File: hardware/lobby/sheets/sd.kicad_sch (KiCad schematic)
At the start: 8 parts, among them J3 Micro_SD_Card_Det, U1 RT9742GGJ5

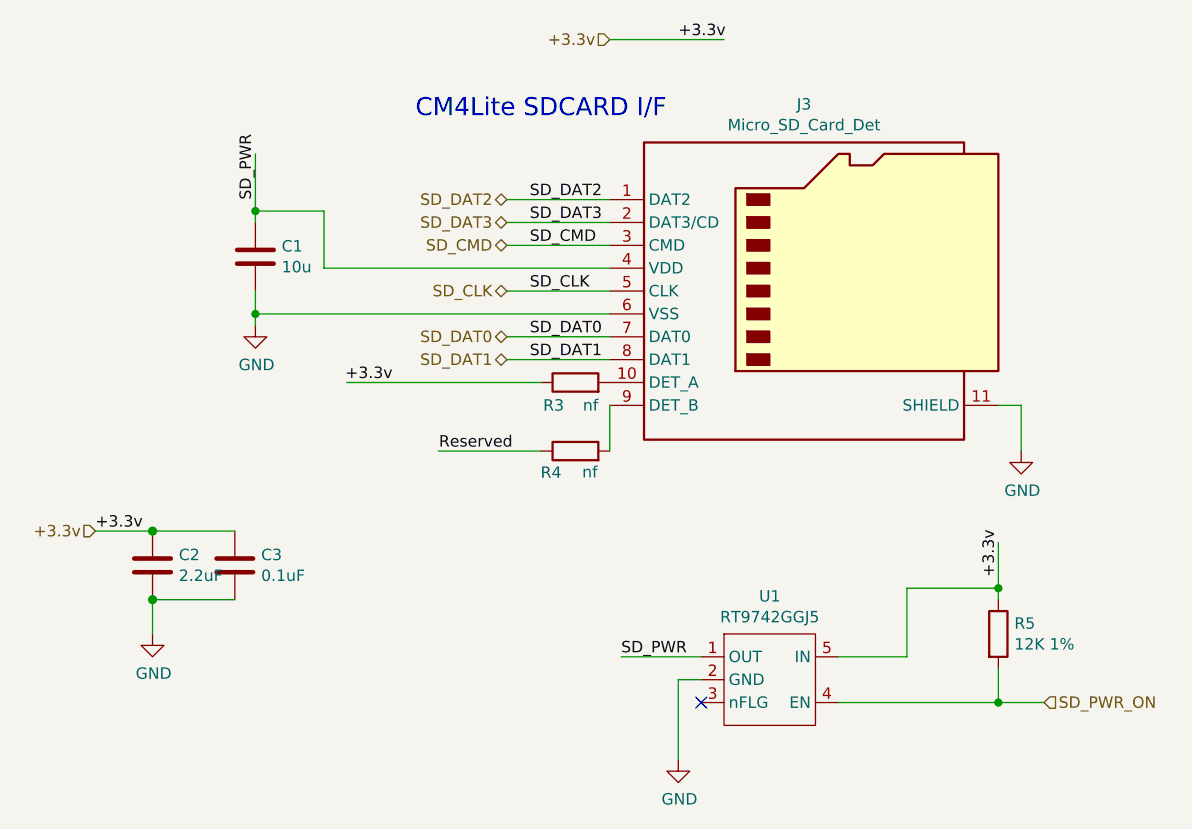
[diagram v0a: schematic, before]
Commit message: update lobby
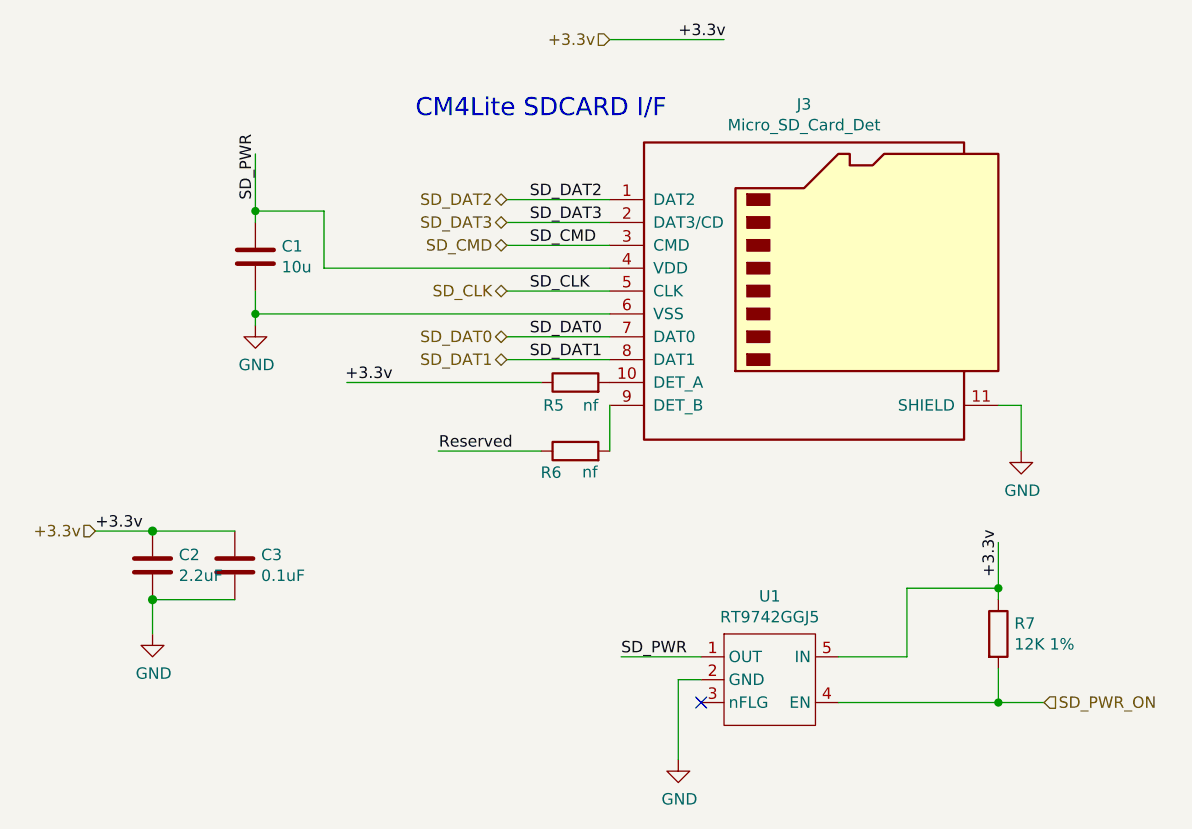
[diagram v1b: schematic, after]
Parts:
- J3: footprint cm4crypto:SDCARD_MOLEX_503398-1892 -> cm4crypto:amphenol-sd-push-pull_114-00841-68
- renumbered R3 to R5, R4 to R6, R5 to R7
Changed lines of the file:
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@@
   (symbol (lib_id "power:GND") (at 86.36 119.38 0) (unit 1)
     (in_bom yes) (on_board yes)
-    (property "Reference" "#PWR056" (id 0) (at 86.36 125.73 0)
+    (property "Reference" "#PWR055" (id 0) (at 86.36 125.73 0)
       (effects (font (size 1.27 1.27)) hide)
     )
@@
   (symbol (lib_id "power:GND") (at 97.79 85.09 0) (unit 1)
     (in_bom yes) (on_board yes)
-    (property "Reference" "#PWR054" (id 0) (at 97.79 91.44 0)
+    (property "Reference" "#PWR053" (id 0) (at 97.79 91.44 0)
       (effects (font (size 1.27 1.27)) hide)
     )
@@
   (symbol (lib_id "power:GND") (at 144.78 133.35 0) (unit 1)
     (in_bom yes) (on_board yes)
-    (property "Reference" "#PWR057" (id 0) (at 144.78 139.7 0)
+    (property "Reference" "#PWR056" (id 0) (at 144.78 139.7 0)
       (effects (font (size 1.27 1.27)) hide)
     )
@@
   (symbol (lib_id "power:GND") (at 182.88 99.06 0) (unit 1)
     (in_bom yes) (on_board yes)
-    (property "Reference" "#PWR055" (id 0) (at 182.88 105.41 0)
+    (property "Reference" "#PWR054" (id 0) (at 182.88 105.41 0)
       (effects (font (size 1.27 1.27)) hide)
     )
@@
   (symbol (lib_id "Device:R") (at 133.35 91.44 90) (unit 1)
     (in_bom yes) (on_board yes)
-    (property "Reference" "R3" (id 0) (at 132.08 93.98 90)
+    (property "Reference" "R5" (id 0) (at 132.08 93.98 90)
       (effects (font (size 1.27 1.27)) (justify left))
     )
@@
       (effects (font (size 1.27 1.27)) hide)
     )
-    (property "Datasheet" "https://fscdn.rohm.com/en/products/databook/datasheet/passive/resistor/chip_resistor/mcr-e.pdf" (id 3) (at 133.35 91.44 0)
+    (property "Datasheet" "~" (id 3) (at 133.35 91.44 0)
       (effects (font (size 1.27 1.27)) hide)
     )
@@
   (symbol (lib_id "Device:R") (at 133.35 99.06 90) (unit 1)
     (in_bom yes) (on_board yes)
-    (property "Reference" "R4" (id 0) (at 131.8006 101.4476 90)
+    (property "Reference" "R6" (id 0) (at 131.8006 101.4476 90)
       (effects (font (size 1.27 1.27)) (justify left))
     )
@@
       (effects (font (size 1.27 1.27)) hide)
     )
-    (property "Datasheet" "https://fscdn.rohm.com/en/products/databook/datasheet/passive/resistor/chip_resistor/mcr-e.pdf" (id 3) (at 133.35 99.06 0)
+    (property "Datasheet" "~" (id 3) (at 133.35 99.06 0)
       (effects (font (size 1.27 1.27)) hide)
     )
@@
   (symbol (lib_id "Device:R") (at 180.34 119.38 0) (unit 1)
     (in_bom yes) (on_board yes)
-    (property "Reference" "R5" (id 0) (at 182.118 118.2116 0)
+    (property "Reference" "R7" (id 0) (at 182.118 118.2116 0)
       (effects (font (size 1.27 1.27)) (justify left))
     )
@@
       (effects (font (size 1.27 1.27)) hide)
     )
-    (property "Datasheet" "https://fscdn.rohm.com/en/products/databook/datasheet/passive/resistor/chip_resistor/mcr-e.pdf" (id 3) (at 180.34 119.38 0)
+    (property "Datasheet" "~" (id 3) (at 180.34 119.38 0)
       (effects (font (size 1.27 1.27)) hide)
     )
@@
       (effects (font (size 1.27 1.27)) hide)
     )
-    (property "Datasheet" "https://search.murata.co.jp/Ceramy/image/img/A01X/G101/ENG/GRM21BR71A106KA73-01.pdf" (id 3) (at 86.36 111.76 0)
+    (property "Datasheet" "~" (id 3) (at 86.36 111.76 0)
       (effects (font (size 1.27 1.27)) hide)
     )
@@
       (effects (font (size 1.27 1.27)) hide)
     )
-    (property "Datasheet" "https://search.murata.co.jp/Ceramy/image/img/A01X/G101/ENG/GRM21BR71A106KA73-01.pdf" (id 3) (at 95.504 111.76 0)
+    (property "Datasheet" "~" (id 3) (at 95.504 111.76 0)
       (effects (font (size 1.27 1.27)) hide)
     )
@@
       (effects (font (size 1.27 1.27)) hide)
     )
-    (property "Datasheet" "https://search.murata.co.jp/Ceramy/image/img/A01X/G101/ENG/GRM21BR71A106KA73-01.pdf" (id 3) (at 97.79 77.47 0)
+    (property "Datasheet" "~" (id 3) (at 97.79 77.47 0)
       (effects (font (size 1.27 1.27)) hide)
     )
@@
     (property "Reference" "J3" (id 0) (at 158.75 60.5282 0))
     (property "Value" "Micro_SD_Card_Det" (id 1) (at 158.75 62.8396 0))
-    (property "Footprint" "cm4crypto:SDCARD_MOLEX_503398-1892" (id 2) (at 212.09 63.5 0)
-      (effects (font (size 1.27 1.27)) hide)
-    )
+    (property "Footprint" "cm4crypto:amphenol-sd-push-pull_114-00841-68" (id 2) (at 212.09 63.5 0)
+      (effects (font (size 1.27 1.27)) hide)
+    )
